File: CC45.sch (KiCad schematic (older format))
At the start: 21 parts, among them J1 AVR-ISP-6, SW1 RESET, U1 ATmega32U4-AU, U2 PRTR5V0U2X, X1 XTAL

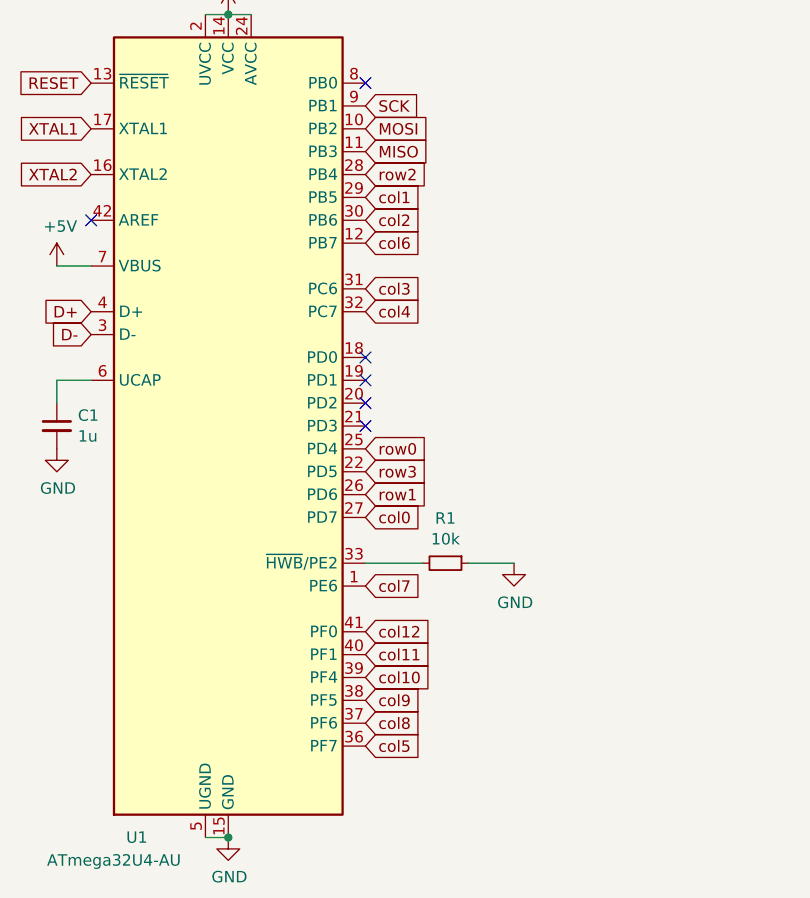
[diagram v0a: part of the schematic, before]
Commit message: v2 update
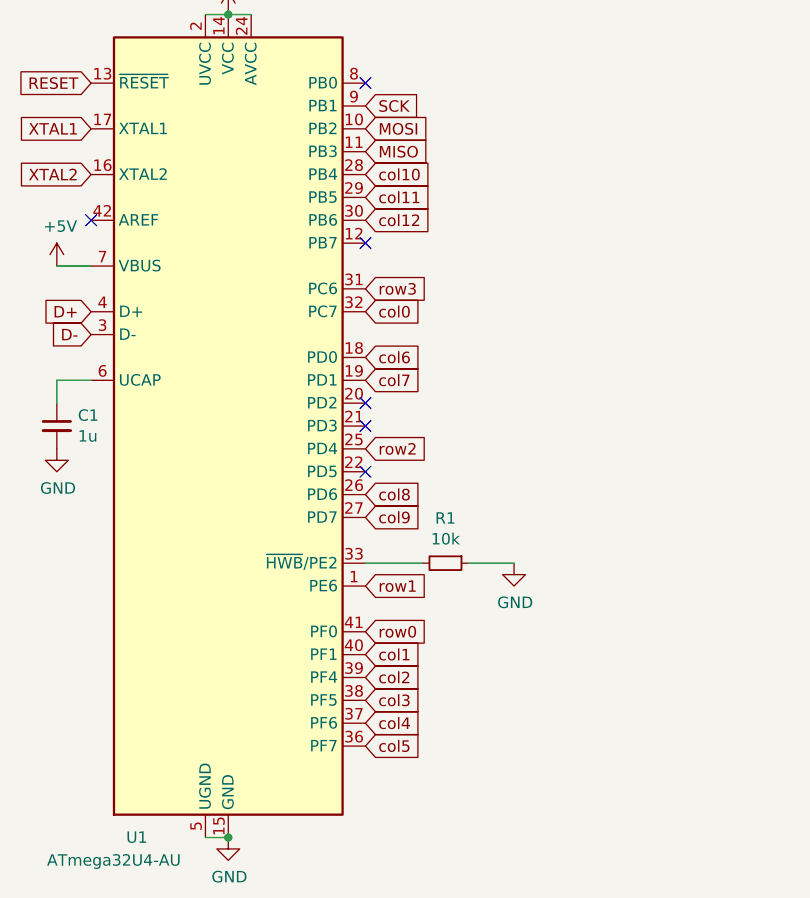
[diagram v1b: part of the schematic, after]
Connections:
- net col0: now also U1.32 (PC7); no longer U1.27 (PD7)
- net col1: now also U1.40 (PF1); no longer U1.29 (PB5)
- net col10: now also U1.28 (PB4); no longer U1.39 (PF4)
- net col11: now also U1.29 (PB5); no longer U1.40 (PF1)
- net col12: now also U1.30 (PB6); no longer U1.41 (PF0)
- net col2: now also U1.39 (PF4); no longer U1.30 (PB6)
- net col3: now also U1.38 (PF5); no longer U1.31 (PC6)
- net col4: now also U1.37 (PF6); no longer U1.32 (PC7)
- net col6: now also U1.18 (PD0); no longer U1.12 (PB7)
- net col7: now also U1.19 (PD1); no longer U1.1 (PE6)
- net col8: now also U1.26 (PD6); no longer U1.37 (PF6)
- net col9: now also U1.27 (PD7); no longer U1.38 (PF5)
- net row0: now also U1.41 (PF0); no longer U1.25 (PD4)
- net row1: now also U1.1 (PE6); no longer U1.26 (PD6)
- net row2: now also U1.25 (PD4); no longer U1.28 (PB4)
- net row3: now also U1.31 (PC6); no longer U1.22 (PD5)
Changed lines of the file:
@@
 Text GLabel 2550 1750 2    50   Input ~ 0
 MISO
-Text GLabel 2550 2150 2    50   Input ~ 0
+Text GLabel 2550 2650 2    50   Input ~ 0
 col6
+Text GLabel 2550 3050 2    50   Input ~ 0
+row2
+Text GLabel 2550 2050 2    50   Input ~ 0
+col12
+Text GLabel 2550 1950 2    50   Input ~ 0
+col11
 Text GLabel 2550 1850 2    50   Input ~ 0
-row2
-Text GLabel 2550 3850 2    50   Input ~ 0
-col12
-Text GLabel 2550 3950 2    50   Input ~ 0
-col11
-Text GLabel 2550 4050 2    50   Input ~ 0
 col10
-Text GLabel 2550 4150 2    50   Input ~ 0
+Text GLabel 2550 3350 2    50   Input ~ 0
 col9
-Text GLabel 2550 4250 2    50   Input ~ 0
+Text GLabel 2550 3250 2    50   Input ~ 0
 col8
-Text GLabel 2550 3650 2    50   Input ~ 0
+Text GLabel 2550 2750 2    50   Input ~ 0
 col7
 Text GLabel 2550 4350 2    50   Input ~ 0
 col5
+Text GLabel 2550 4250 2    50   Input ~ 0
+col4
+Text GLabel 2550 4150 2    50   Input ~ 0
+col3
+Text GLabel 2550 4050 2    50   Input ~ 0
+col2
+Text GLabel 2550 3950 2    50   Input ~ 0
+col1
 Text GLabel 2550 2450 2    50   Input ~ 0
-col4
+col0
+Text GLabel 2550 3850 2    50   Input ~ 0
+row0
+Text GLabel 2550 3650 2    50   Input ~ 0
+row1
 Text GLabel 2550 2350 2    50   Input ~ 0
-col3
-Text GLabel 2550 2050 2    50   Input ~ 0
-col2
-Text GLabel 2550 1950 2    50   Input ~ 0
-col1
-Text GLabel 2550 3350 2    50   Input ~ 0
-col0
-Text GLabel 2550 3050 2    50   Input ~ 0
-row0
-Text GLabel 2550 3250 2    50   Input ~ 0
-row1
-Text GLabel 2550 3150 2    50   Input ~ 0
 row3
-NoConn ~ 2550 2650
-NoConn ~ 2550 2750
+NoConn ~ 2550 2150
+NoConn ~ 2550 3150
 NoConn ~ 2550 2850
 NoConn ~ 2550 2950
